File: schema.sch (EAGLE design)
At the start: 10 parts, among them J1 DCJ0202, X1 BU-SMA-G

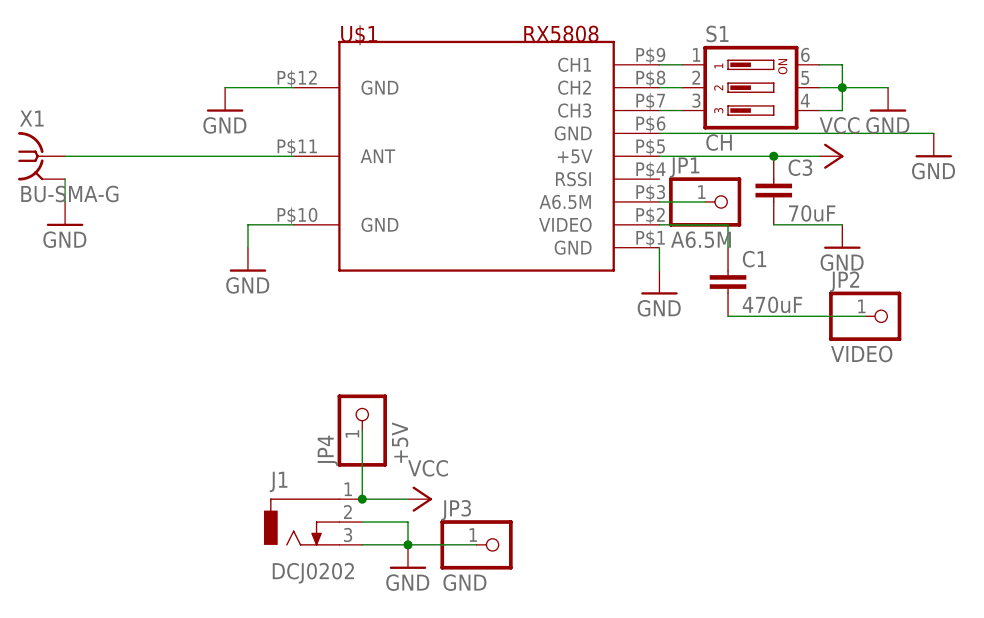
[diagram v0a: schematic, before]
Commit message: Fixed pin switching issue and various
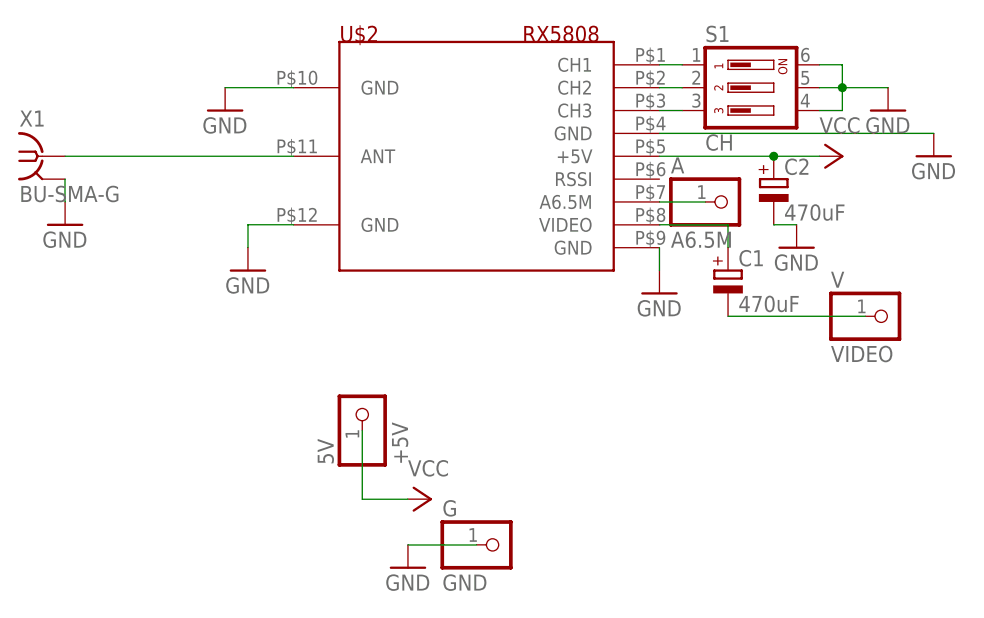
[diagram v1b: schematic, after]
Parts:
- removed C3: 70uF, resistor:C-EU025-025X050
- removed J1: DCJ0202, con-jack:DCJ0202
- removed U$1: RX5808, hi-link:RX5808
- added C2: 470uF, resistor:CPOL-EUE3.5-8
- added U$2: RX5808, custom-parts:RX5808
- C1: device resistor:C-EU025-025X050 -> resistor:CPOL-EUE3.5-8
- renumbered JP1 to A, JP2 to V, JP3 to G, JP4 to 5V
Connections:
- removed net N$1: U$1.ANT, X1.1
- new net ANTENA: U$2.ANT, X1.1
- net AUDIO: now also U$2.A6.5M; no longer U$1.A6.5M
- net CH1: now also U$2.CH1; no longer U$1.CH1
- net CH2: now also U$2.CH2; no longer U$1.CH2
- net CH3: now also U$2.CH3; no longer U$1.CH3
- net GND: now also C2.-, U$2.GND@1, U$2.GND@2, U$2.GND@3, U$2.GND@4; no longer C3.2, J1.2, J1.3, U$1.GND@1, U$1.GND@2, U$1.GND@3, U$1.GND@4
- net VCC: now also C2.+, U$2.+5V; no longer C3.1, J1.1, U$1.+5V
- net VIDEO_IN: now also C1.+, U$2.VIDEO; no longer C1.1, U$1.VIDEO
- net VIDEO_OUT: now also C1.-; no longer C1.2
